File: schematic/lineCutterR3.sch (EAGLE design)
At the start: 62 parts, among them IC2 MC33269ST-3.3T3, J1 10118192-0001LF, Q1 AO4576, Q2 AO4576, Q4 AO4576, Q5 DMG2305, SW1 KMR2, U1 MS560702BA03-50, U2 MDBT50Q, U3 S25FL128SDPMFIG13S03016, U4 ACS711KEXLT-31AB-T, U6 ICM-20602, X1 2x5 0.05", Y2 32.768

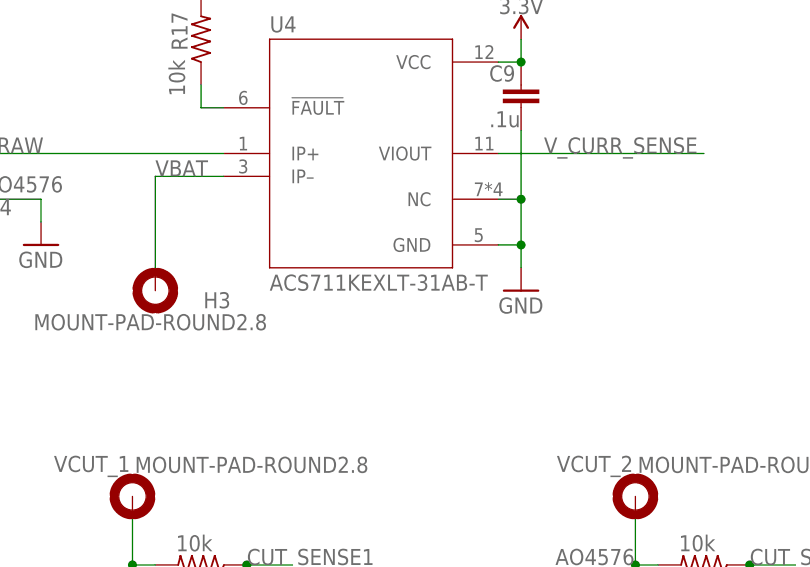
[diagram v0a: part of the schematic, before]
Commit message: Final board stuff
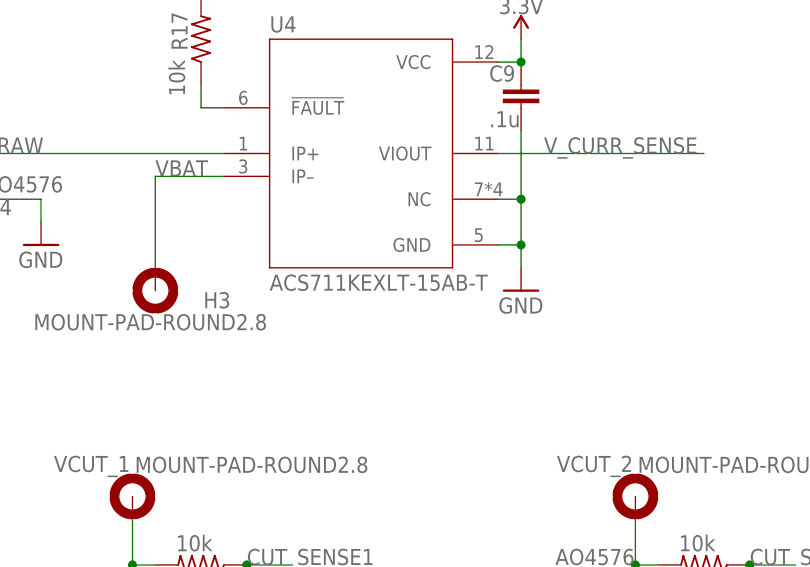
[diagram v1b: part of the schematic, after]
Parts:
- U4: value ACS711KEXLT-31AB-T -> ACS711KEXLT-15AB-T
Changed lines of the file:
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@@
 <part name="GND22" library="supply1" library_urn="urn:adsk.eagle:library:371" deviceset="GND" device=""/>
 <part name="SUPPLY10" library="SparkFun-PowerSymbols" deviceset="3.3V" device=""/>
-<part name="U4" library="Line Cutter COTS" deviceset="ACS711KEXLT-31AB-T" device=""/>
+<part name="U4" library="Line Cutter COTS" deviceset="ACS711KEXLT-31AB-T" device="" value="ACS711KEXLT-15AB-T"/>
 <part name="D2" library="SparkFun-LED" deviceset="SUNLED" device="SMD1" value="XZM2CRKM2DGFBB45SCCB"/>
 <part name="GND7" library="supply1" library_urn="urn:adsk.eagle:library:371" deviceset="GND" device=""/>
